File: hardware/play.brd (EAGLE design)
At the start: 22.9 x 40 mm, 14 parts, among them T1 BC547, T2 BC547, T3 BC547, T4 BC547

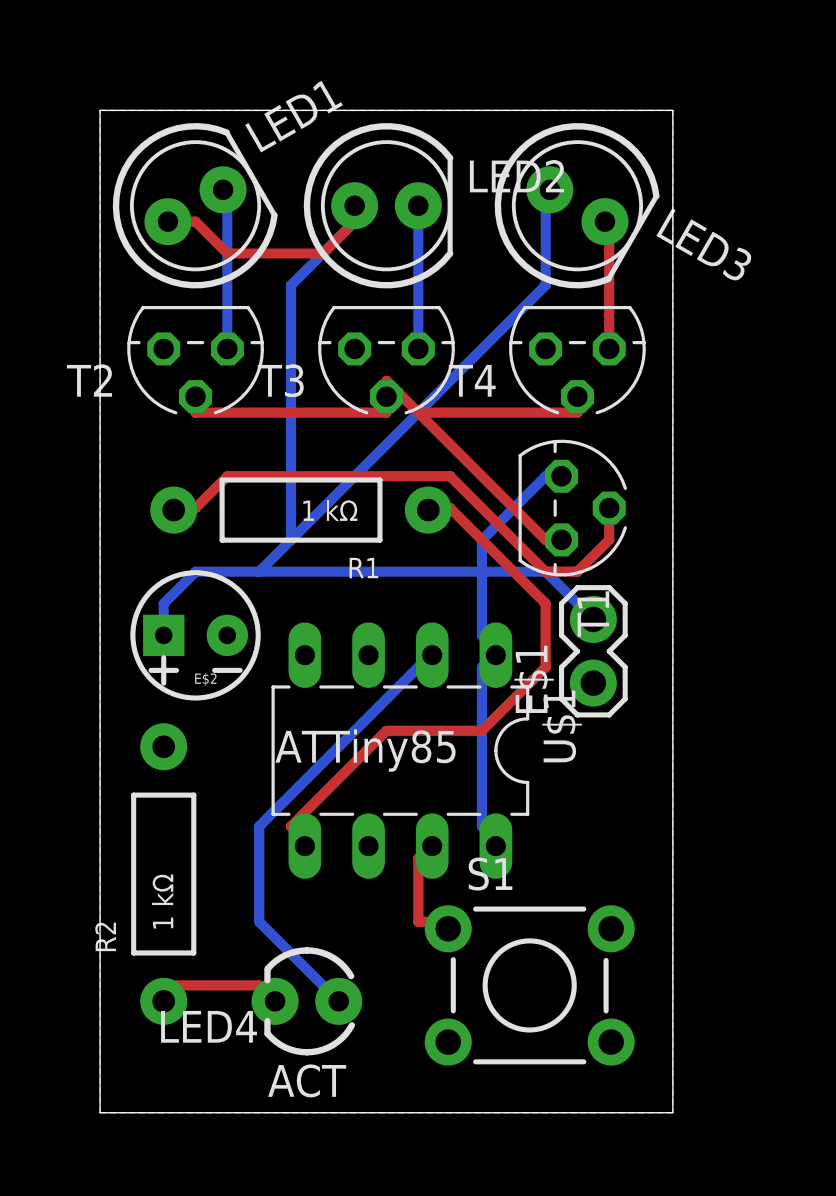
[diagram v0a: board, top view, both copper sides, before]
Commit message: New hardware PCB design, with signal connector
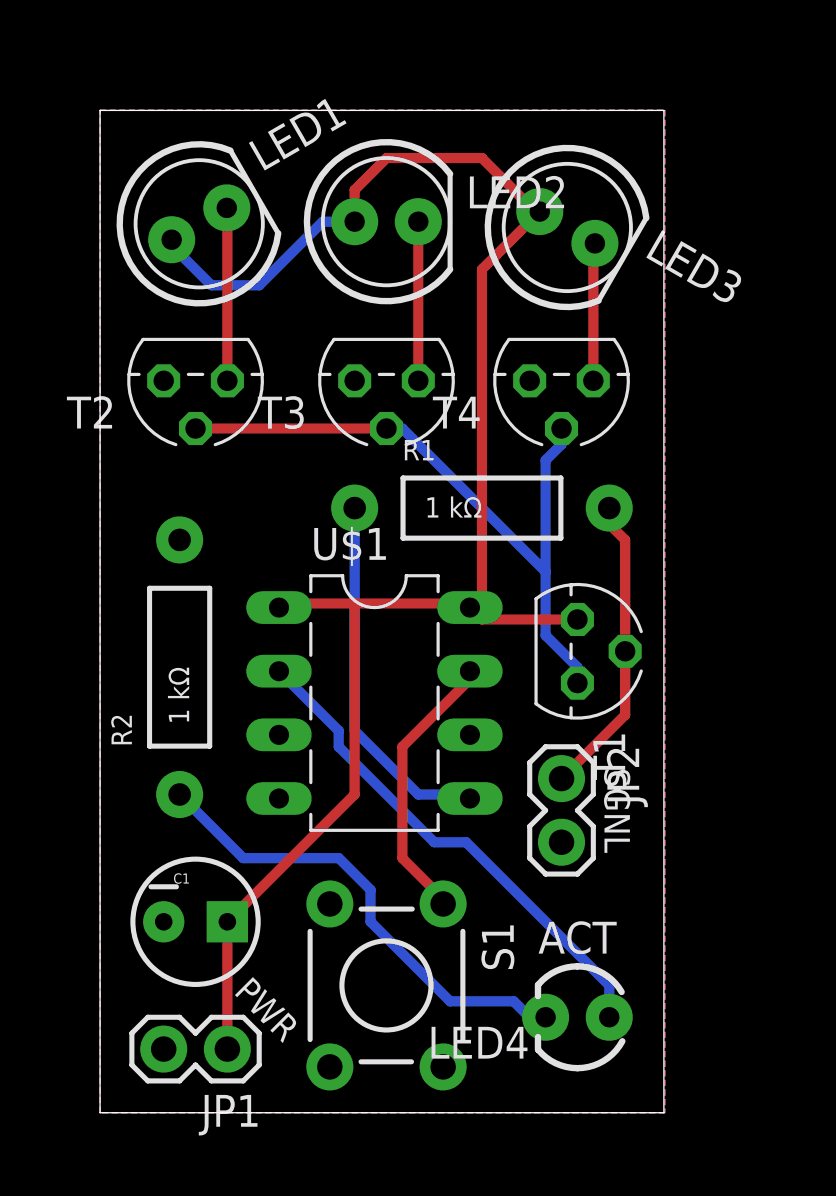
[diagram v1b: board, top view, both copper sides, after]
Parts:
- removed E$1: (no value), SparkFun-Connectors:1X02
- removed E$2: (no value), SparkFun-Capacitors:CPOL-RADIAL-10UF-25V-KIT
- added C1: 10µF, SparkFun-Capacitors:CPOL-RADIAL-10UF-25V
- added JP1, JP2: M02PTH, SparkFun-Connectors:1X02
- moved LED4 10.8 mm to (19.1, 3.81)
- moved R2 8.28 mm to (3.17, 17.8)
- moved R1 7.22 mm to (15.2, 24.1), turned to 0 degrees
- moved T1 5.75 mm to (19.1, 18.4)
- moved S1 5.71 mm to (11.4, 5.08), turned to 270 degrees
- moved U$1 2.16 mm to (10.9, 16.4), turned to 0 degrees
- moved T4 1.42 mm to (18.4, 29.2)
- moved T2 1.27 mm to (3.81, 29.2)
- moved T3 1.27 mm to (11.4, 29.2)
- moved LED3 0.96 mm to (18.6, 35.3)
- moved LED1 0.73 mm to (3.96, 35.5)
- moved LED2 0.63 mm to (11.4, 35.6)
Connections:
- net GND: now also C1.2, JP1.2, JP2.2; no longer E$1.1, E$2.2
- net N$2: now also JP2.1
- net VCC: now also C1.1, JP1.1; no longer E$1.2, E$2.1
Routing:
- net N$9: track 5.34 -> 19.0 mm
- net VCC: track 80.6 -> 68.4 mm
- net N$2: track 21.3 -> 12.1 mm
- net N$1: track 22.6 -> 14.6 mm
- net N$5: track 4.83 -> 11.0 mm
- net N$8: track 18.0 -> 20.0 mm
- net N$3: track 26.1 -> 27.3 mm
- net N$6: track 5.71 -> 6.35 mm
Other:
- board size 22.9 x 40 mm -> 22.5 x 40 mm
- board text added: "(this is not a bomb)"
- board text added: "PWR"
- board text added: "SGNL"
- board text added: "batch"
- board text removed: "ATTiny85"
